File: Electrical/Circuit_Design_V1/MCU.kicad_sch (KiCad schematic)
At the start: 16 parts, among them SW1 SW_Push, SW2 SW_Push, U1 STM32G474RETx

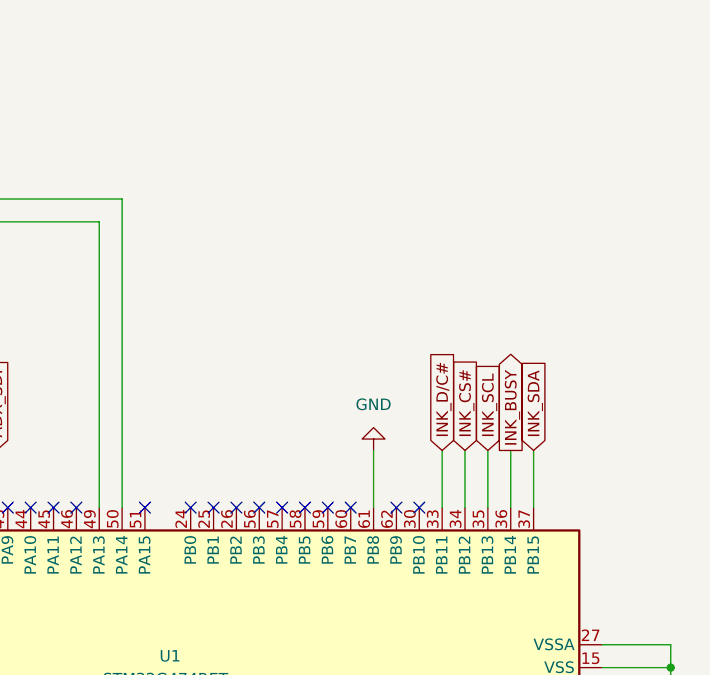
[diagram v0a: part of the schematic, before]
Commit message: Adding pots.
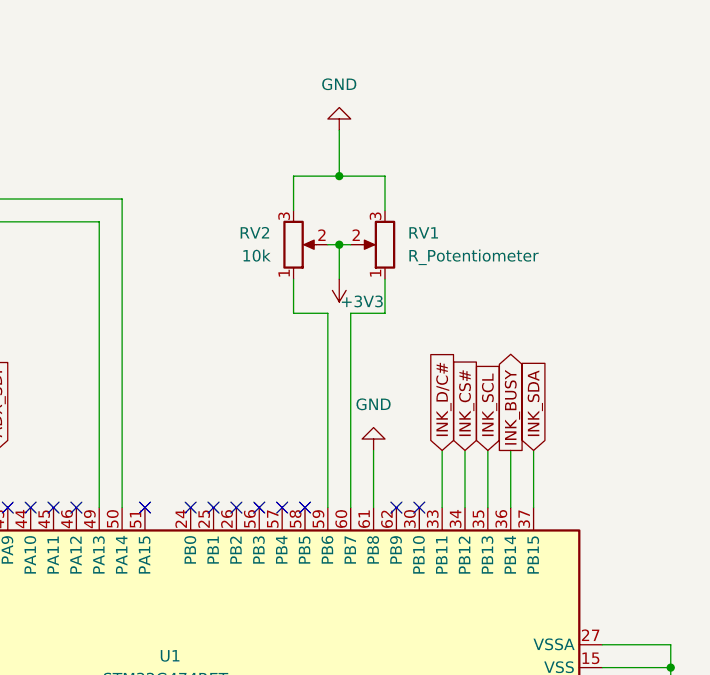
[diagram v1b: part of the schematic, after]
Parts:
- added RV1: R_Potentiometer, Etchasketch_Footprints:Potentiometer, symbol Device:R_Potentiometer
- added RV2: 10k, Etchasketch_Footprints:Potentiometer, symbol Device:R_Potentiometer
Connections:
- net +3V3: now also RV1.2, RV2.2
- net GND: now also RV1.3, RV2.3
- net at U1.59 (PB6): now also RV2.1
- net at U1.60 (PB7): now also RV1.1
- no-connect marks 35 -> 33
